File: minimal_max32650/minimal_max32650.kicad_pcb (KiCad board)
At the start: 4 copper layers, 51.6 x 34.3 mm, 57 parts, among them J1 FTSH-105-01-L-DV-K, Q1 50 V, Q2 50 V, U1 ADT75BRMZ, U2 MX25U6432FZNI02, U3 MAX32650GCE+, U4 MAXQ1065GTC+, U5 ADP225ACPZ-R7

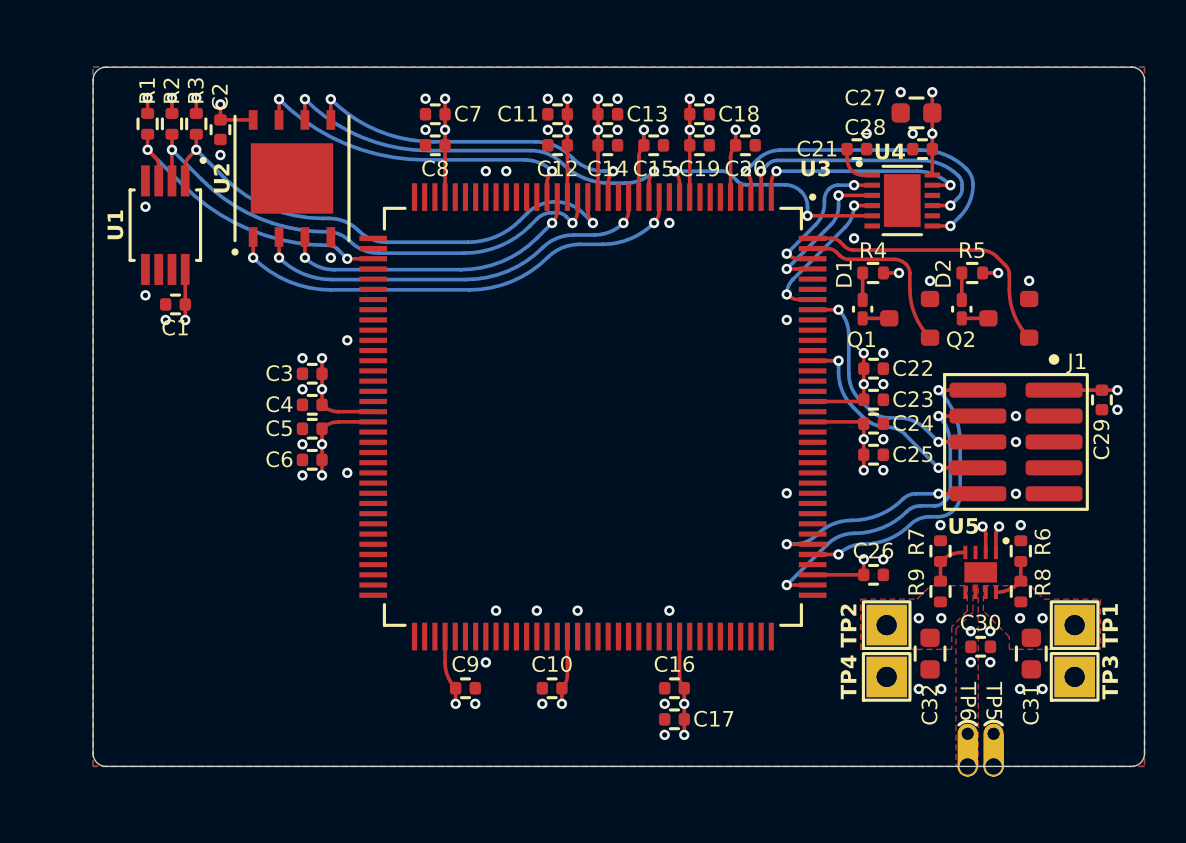
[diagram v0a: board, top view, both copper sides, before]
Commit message: development backup
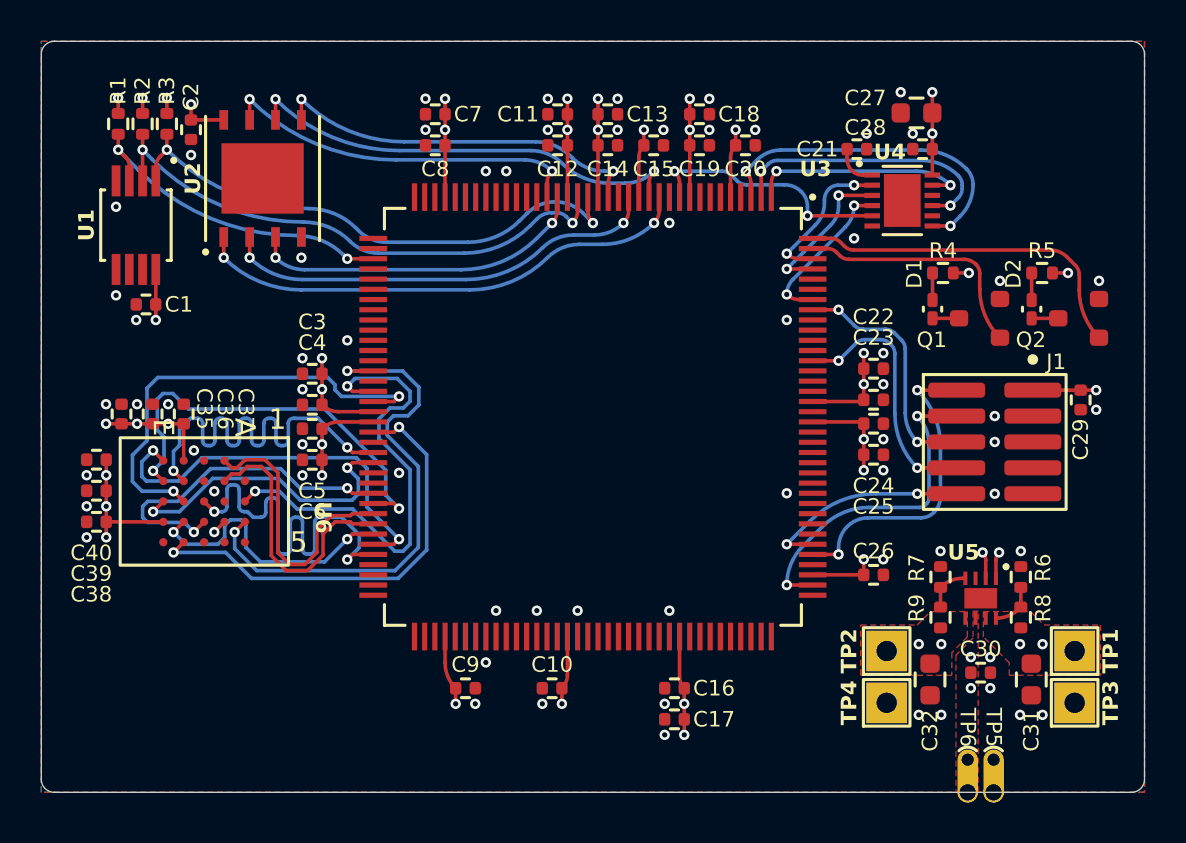
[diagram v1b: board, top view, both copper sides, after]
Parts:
- added C35: 100 nF, capacitor_footprints:C_0402_1005Metric, F.Cu at (142.7, 90.3)
- added C36: 100 nF, capacitor_footprints:C_0402_1005Metric, F.Cu at (144.2, 90.3)
- added C37: 1 µF, capacitor_footprints:C_0402_1005Metric, F.Cu at (145.7, 90.3)
- added C38: 1 µF, capacitor_footprints:C_0402_1005Metric, F.Cu at (141.4, 95.6)
- added C39: 100 nF, capacitor_footprints:C_0402_1005Metric, F.Cu at (141.4, 94.1)
- added C40: 100 nF, capacitor_footprints:C_0402_1005Metric, F.Cu at (141.4, 92.5)
- added U6: S80KS5122GABHM020, infineon_footprints:PG-BGA-24-801, F.Cu at (146.7, 94.6)
- moved D1 3.43 mm to (182.4, 85.1)
- moved D2 3.43 mm to (187.3, 85.1)
- moved Q1 3.43 mm to (184.7, 85.6)
- moved Q2 3.43 mm to (189.6, 85.6)
- moved R4 3.43 mm to (183.0, 83.4)
- moved R5 3.43 mm to (187.8, 83.4)
- moved R1 1.44 mm to (142.5, 76.1)
- moved R2 1.44 mm to (143.7, 76.1)
- moved R3 1.44 mm to (144.9, 76.1)
- moved U1 1.44 mm to (143.4, 81.0)
- moved U2 1.44 mm to (149.6, 78.7)
- moved C1 1.44 mm to (143.9, 84.9)
- moved C2 1.44 mm to (146.1, 76.3)
- moved R8 1.27 mm to (186.8, 100.3)
- moved R9 1.27 mm to (182.8, 100.3)
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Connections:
- U3 pad 44: unconnected-(U2-P3.0-Pad44) -> /CS1__P3.0
- U3 pad 50: unconnected-(U2-P1.10-Pad50) -> /RESET__P1.10
- U3 pad 52: unconnected-(U2-P1.11-Pad52) -> /CS0__P1.11
- U3 pad 53: unconnected-(U2-P1.12-Pad53) -> /D0__P1.12
- U3 pad 56: unconnected-(U2-P1.13-Pad56) -> /D4__P1.13
- U3 pad 58: unconnected-(U2-P1.15-Pad58) -> /D1__P1.15
- U3 pad 59: unconnected-(U2-P1.16-Pad59) -> /D5__P1.16
- U3 pad 62: unconnected-(U2-P1.19-Pad62) -> /D2__P1.19
- U3 pad 63: unconnected-(U2-P1.18-Pad63) -> /D6__P1.18
- U3 pad 64: unconnected-(U2-~{HYP_CLK}-Pad64) -> /CLK_N
- U3 pad 65: unconnected-(U2-HYP_CLK-Pad65) -> /CLK_P
- U3 pad 66: unconnected-(U2-P1.20-Pad66) -> /D3__P1.20
- U3 pad 67: unconnected-(U2-P1.21-Pad67) -> /D7__P1.21
- U3 pad 68: unconnected-(U2-P1.14-Pad68) -> /RWDS__P1.14
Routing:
- net /D1__P1.15: track 0.00 -> 26.8 mm, vias 0 -> 2
- net /RESET__P1.10: track 0.00 -> 26.1 mm, vias 0 -> 2
- net /CS0__P1.11: track 0.00 -> 23.7 mm, vias 0 -> 2
- net /D0__P1.12: track 0.00 -> 22.3 mm, vias 0 -> 2
- net /D4__P1.13: track 0.00 -> 22.2 mm, vias 0 -> 2
- net /RWDS__P1.14: track 0.00 -> 21.3 mm, vias 0 -> 2
- net /D6__P1.18: track 0.00 -> 21.0 mm, vias 0 -> 2
- net /D7__P1.21: track 0.00 -> 19.5 mm, vias 0 -> 2
- net /D2__P1.19: track 0.00 -> 16.6 mm, vias 0 -> 2
- net /D5__P1.16: track 0.00 -> 14.9 mm, vias 0 -> 2
- net /CLK_N: track 0.00 -> 13.7 mm
- net /D3__P1.20: track 0.00 -> 13.7 mm, vias 0 -> 2
- net /CLK_P: track 0.00 -> 13.6 mm
- net /1V8: track 33.0 -> 45.9 mm, vias 15 -> 22
- net /LED2: track 8.69 -> 12.1 mm
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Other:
- board size 51.6 x 34.3 mm -> 54.1 x 36.8 mm
